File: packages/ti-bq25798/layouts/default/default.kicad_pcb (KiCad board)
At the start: 2 copper layers, 7 parts

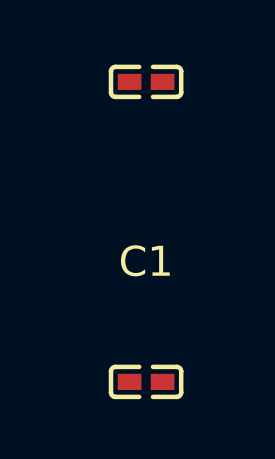
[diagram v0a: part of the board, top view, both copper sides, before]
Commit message: BQ25798
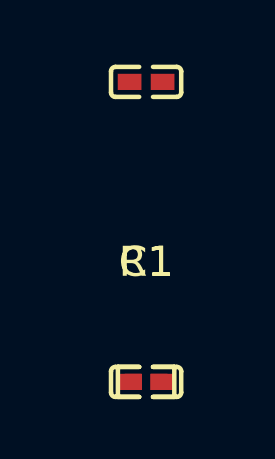
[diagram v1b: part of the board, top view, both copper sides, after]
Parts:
- added R1: 390Ω ±1% 100mW, PANASONIC_ERJ2RKF3900X:R0402, F.Cu at (0.00, 0.00)
